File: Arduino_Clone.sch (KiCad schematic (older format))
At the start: 11 parts

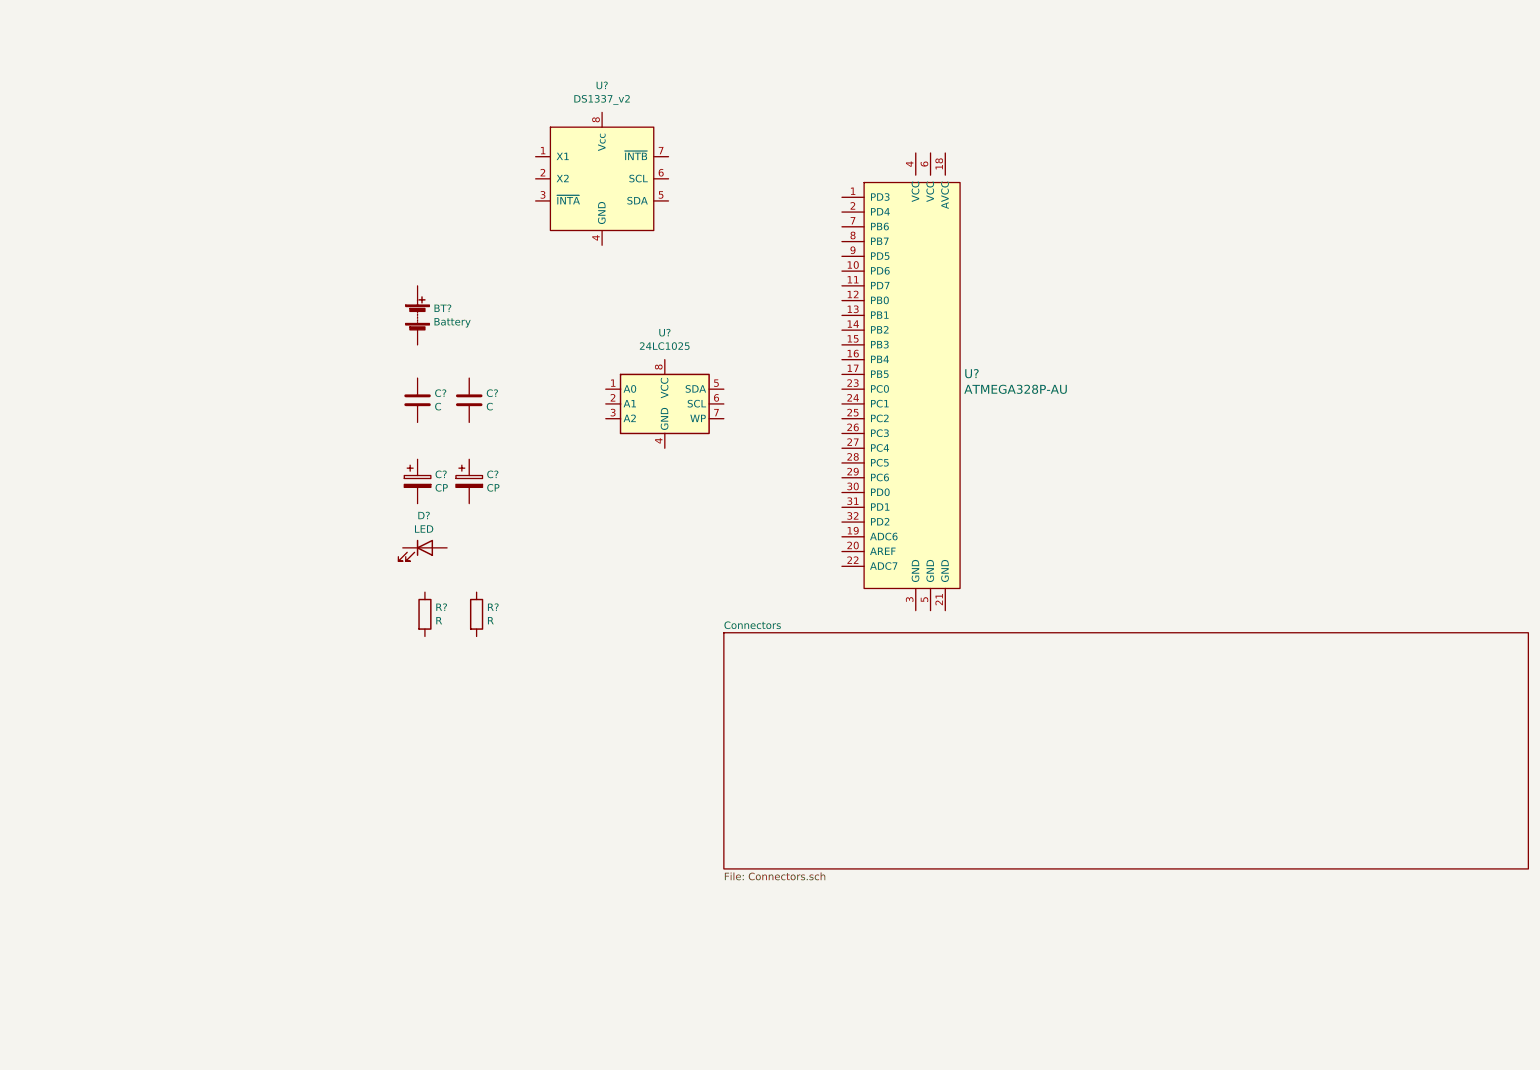
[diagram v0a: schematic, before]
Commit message: Added footprint associations.
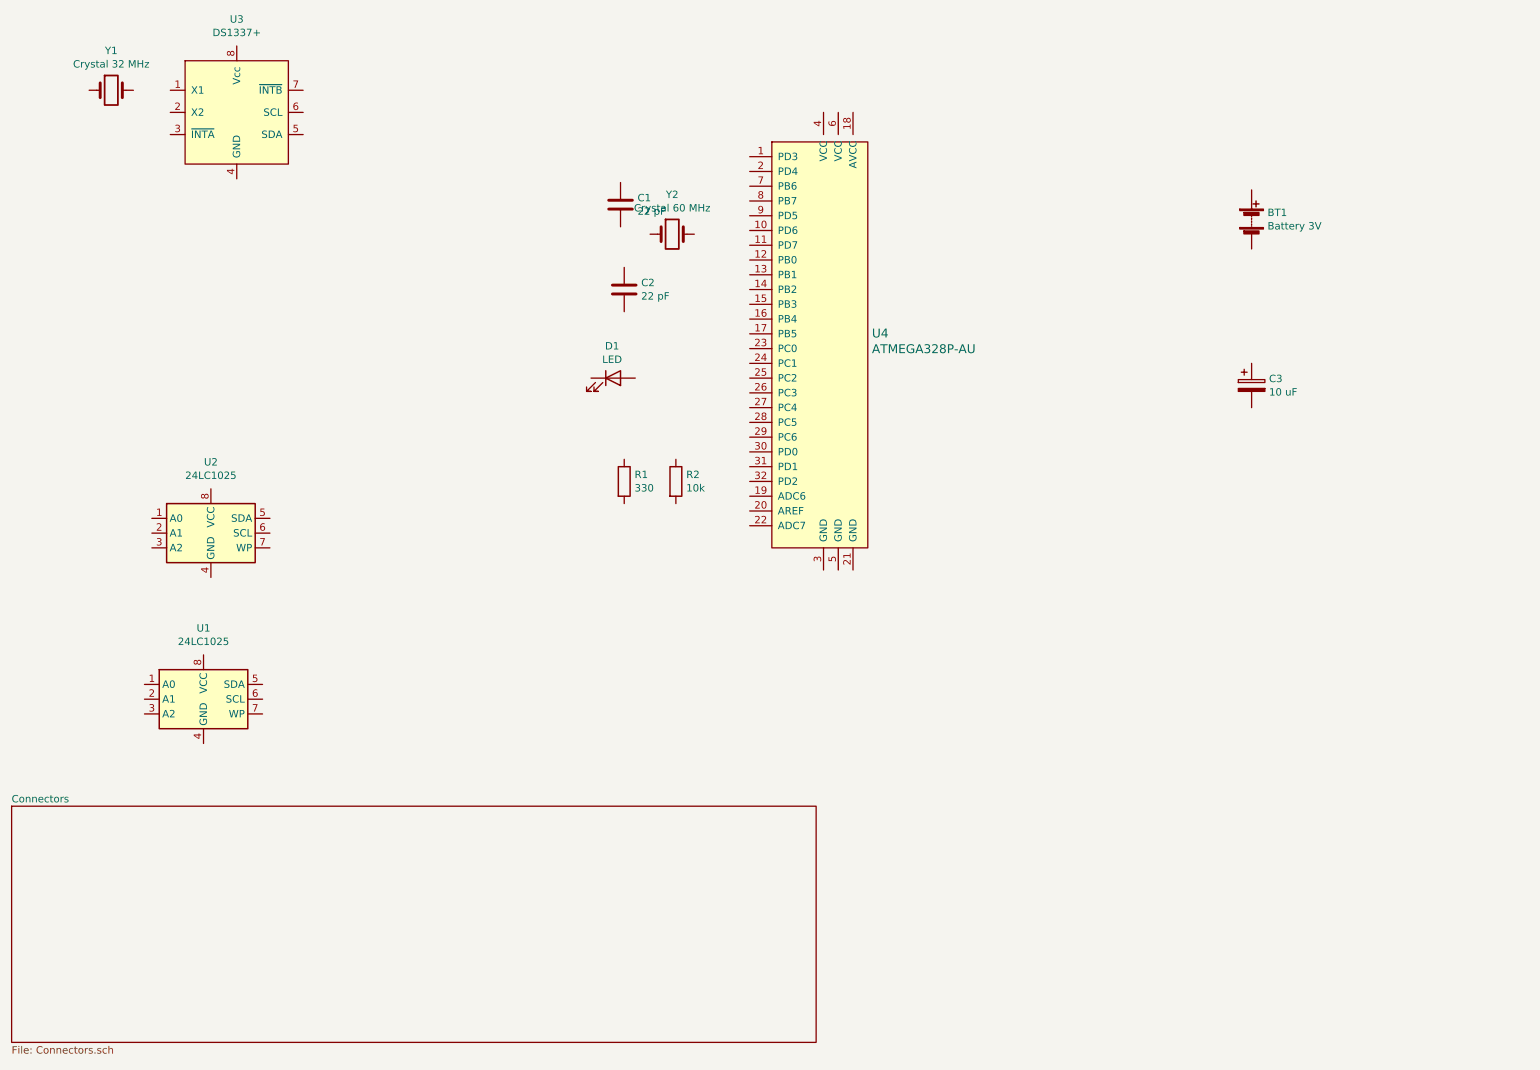
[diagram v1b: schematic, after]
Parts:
- removed C?: CP, symbol Device:CP
- added U2: 24LC1025, Footprints:SOIC-8_3.9mmX4.9mm, symbol Memory_EEPROM:24LC1025
- added Y1: Crystal 32 MHz, Crystal:Crystal_SMD_MicroCrystal_CC7V-T1A-2Pin_3.2x1.5mm_HandSoldering, symbol Device:Crystal
- added Y2: Crystal 60 MHz, Crystal:Crystal_SMD_5032-2Pin_5.0x3.2mm_HandSoldering, symbol Device:Crystal
- BT1: renamed from BT?; value Battery -> Battery 3V; footprint (none) -> Capacitor_SMD:C_0805_2012Metric
- C1, C2: renamed from C?; value C -> 22 pF; footprint (none) -> Capacitor_SMD:C_0805_2012Metric_Pad1.18x1.45mm_HandSolder
- C3: renamed from C?; value CP -> 10 uF; footprint (none) -> Capacitor_SMD:C_0805_2012Metric_Pad1.18x1.45mm_HandSolder
- D1: renamed from D?; footprint (none) -> LED_SMD:LED_0805_2012Metric_Pad1.15x1.40mm_HandSolder
- R1: renamed from R?; value R -> 330; footprint (none) -> Resistor_SMD:R_0805_2012Metric_Pad1.20x1.40mm_HandSolder
- R2: renamed from R?; value R -> 10k; footprint (none) -> Resistor_SMD:R_0805_2012Metric_Pad1.20x1.40mm_HandSolder
- U1: renamed from U?; footprint (none) -> Footprints:SOIC-8_3.9mmX4.9mm
- U3: renamed from U?; value DS1337_v2 -> DS1337+; footprint (none) -> Package_SO:SOIC-8_3.9x4.9mm_P1.27mm
- gave numbers to parts that had none: 1
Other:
- moved on the sheet: BT1, C1, C2, C3, D1, R1, R2, U1, U3, U4
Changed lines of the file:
@@
 $EndDescr
 $Comp
-L Device:Battery BT?
+L Device:Battery BT1
 U 1 1 6016CB0C
-P 3625 2700
-F 0 "BT?" H 3733 2746 50  0000 L CNN
-F 1 "Battery" H 3733 2655 50  0000 L CNN
-F 2 "" V 3625 2760 50  0001 C CNN
-F 3 "~" V 3625 2760 50  0001 C CNN
-	1    3625 2700
+P 9275 2050
+F 0 "BT1" H 9383 2096 50  0000 L CNN
+F 1 "Battery 3V" H 9383 2005 50  0000 L CNN
+F 2 "Capacitor_SMD:C_0805_2012Metric" V 9275 2110 50  0001 C CNN
+F 3 "~" V 9275 2110 50  0001 C CNN
+	1    9275 2050
 	1    0    0    -1
 $EndComp
 $Comp
-L Device:C C?
+L Device:C C1
 U 1 1 6016DE4E
-P 3625 3275
-F 0 "C?" H 3740 3321 50  0000 L CNN
-F 1 "C" H 3740 3230 50  0000 L CNN
-F 2 "" H 3663 3125 50  0001 C CNN
-F 3 "~" H 3625 3275 50  0001 C CNN
-	1    3625 3275
+P 5000 1950
+F 0 "C1" H 5115 1996 50  0000 L CNN
+F 1 "22 pF" H 5115 1905 50  0000 L CNN
+F 2 "Capacitor_SMD:C_0805_2012Metric_Pad1.18x1.45mm_HandSolder" H 5038 1800 50  0001 C CNN
+F 3 "~" H 5000 1950 50  0001 C CNN
+	1    5000 1950
 	1    0    0    -1
 $EndComp
 $Comp
-L Device:C C?
+L Device:C C2
 U 1 1 6016E4DC
-P 3975 3275
-F 0 "C?" H 4090 3321 50  0000 L CNN
-F 1 "C" H 4090 3230 50  0000 L CNN
-F 2 "" H 4013 3125 50  0001 C CNN
-F 3 "~" H 3975 3275 50  0001 C CNN
-	1    3975 3275
+P 5025 2525
+F 0 "C2" H 5140 2571 50  0000 L CNN
+F 1 "22 pF" H 5140 2480 50  0000 L CNN
+F 2 "Capacitor_SMD:C_0805_2012Metric_Pad1.18x1.45mm_HandSolder" H 5063 2375 50  0001 C CNN
+F 3 "~" H 5025 2525 50  0001 C CNN
+	1    5025 2525
 	1    0    0    -1
 $EndComp
 $Comp
-L Device:CP C?
+L Device:CP C3
 U 1 1 6016E8E4
-P 3625 3825
-F 0 "C?" H 3743 3871 50  0000 L CNN
-F 1 "CP" H 3743 3780 50  0000 L CNN
-F 2 "" H 3663 3675 50  0001 C CNN
-F 3 "~" H 3625 3825 50  0001 C CNN
-	1    3625 3825
+P 9275 3175
+F 0 "C3" H 9393 3221 50  0000 L CNN
+F 1 "10 uF" H 9393 3130 50  0000 L CNN
+F 2 "Capacitor_SMD:C_0805_2012Metric_Pad1.18x1.45mm_HandSolder" H 9313 3025 50  0001 C CNN
+F 3 "~" H 9275 3175 50  0001 C CNN
+	1    9275 3175
 	1    0    0    -1
 $EndComp
 $Comp
-L Device:CP C?
-U 1 1 6016ED96
-P 3975 3825
-F 0 "C?" H 4093 3871 50  0000 L CNN
-F 1 "CP" H 4093 3780 50  0000 L CNN
-F 2 "" H 4013 3675 50  0001 C CNN
-F 3 "~" H 3975 3825 50  0001 C CNN
-	1    3975 3825
+L Device:LED D1
+U 1 1 6016F1E9
+P 4950 3125
+F 0 "D1" H 4943 3342 50  0000 C CNN
+F 1 "LED" H 4943 3251 50  0000 C CNN
+F 2 "LED_SMD:LED_0805_2012Metric_Pad1.15x1.40mm_HandSolder" H 4950 3125 50  0001 C CNN
+F 3 "~" H 4950 3125 50  0001 C CNN
+	1    4950 3125
 	1    0    0    -1
 $EndComp
 $Comp
-L Device:LED D?
-U 1 1 6016F1E9
-P 3675 4275
-F 0 "D?" H 3668 4492 50  0000 C CNN
-F 1 "LED" H 3668 4401 50  0000 C CNN
-F 2 "" H 3675 4275 50  0001 C CNN
-F 3 "~" H 3675 4275 50  0001 C CNN
-	1    3675 4275
+L Device:R R1
+U 1 1 6016F7B9
+P 5025 3825
+F 0 "R1" H 5095 3871 50  0000 L CNN
+F 1 "330" H 5095 3780 50  0000 L CNN
+F 2 "Resistor_SMD:R_0805_2012Metric_Pad1.20x1.40mm_HandSolder" V 4955 3825 50  0001 C CNN
+F 3 "~" H 5025 3825 50  0001 C CNN
+	1    5025 3825
 	1    0    0    -1
 $EndComp
 $Comp
-L Device:R R?
-U 1 1 6016F7B9
-P 3675 4725
-F 0 "R?" H 3745 4771 50  0000 L CNN
-F 1 "R" H 3745 4680 50  0000 L CNN
-F 2 "" V 3605 4725 50  0001 C CNN
-F 3 "~" H 3675 4725 50  0001 C CNN
-	1    3675 4725
+L Device:R R2
+U 1 1 6016FC62
+P 5375 3825
+F 0 "R2" H 5445 3871 50  0000 L CNN
+F 1 "10k" H 5445 3780 50  0000 L CNN
+F 2 "Resistor_SMD:R_0805_2012Metric_Pad1.20x1.40mm_HandSolder" V 5305 3825 50  0001 C CNN
+F 3 "~" H 5375 3825 50  0001 C CNN
+	1    5375 3825
 	1    0    0    -1
 $EndComp
 $Comp
-L Device:R R?
-U 1 1 6016FC62
-P 4025 4725
-F 0 "R?" H 4095 4771 50  0000 L CNN
-F 1 "R" H 4095 4680 50  0000 L CNN
-F 2 "" V 3955 4725 50  0001 C CNN
-F 3 "~" H 4025 4725 50  0001 C CNN
-	1    4025 4725
+L Memory_EEPROM:24LC1025 U1
+U 1 1 60170312
+P 2175 5300
+F 0 "U1" H 2175 5781 50  0000 C CNN
+F 1 "24LC1025" H 2175 5690 50  0000 C CNN
+F 2 "Footprints:SOIC-8_3.9mmX4.9mm" H 2175 5300 50  0001 C CNN
+F 3 "http://ww1.microchip.com/downloads/en/DeviceDoc/21941B.pdf" H 2175 5300 50  0001 C CNN
+	1    2175 5300
 	1    0    0    -1
 $EndComp
 $Comp
-L Memory_EEPROM:24LC1025 U?
-U 1 1 60170312
-P 5300 3300
-F 0 "U?" H 5300 3781 50  0000 C CNN
-F 1 "24LC1025" H 5300 3690 50  0000 C CNN
-F 2 "" H 5300 3300 50  0001 C CNN
-F 3 "http://ww1.microchip.com/downloads/en/DeviceDoc/21941B.pdf" H 5300 3300 50  0001 C CNN
-	1    5300 3300
-	1    0    0    -1
-$EndComp
-$Comp
-L dk_Embedded-Microcontrollers:ATMEGA328P-AU U?
+L dk_Embedded-Microcontrollers:ATMEGA328P-AU U4
 U 1 1 601716D4
-P 7000 3200
-F 0 "U?" H 7328 3303 60  0000 L CNN
-F 1 "ATMEGA328P-AU" H 7328 3197 60  0000 L CNN
-F 2 "digikey-footprints:TQFP-32_7x7mm" H 7200 3400 60  0001 L CNN
-F 3 "http://www.microchip.com/mymicrochip/filehandler.aspx?ddocname=en608326" H 7200 3500 60  0001 L CNN
-F 4 "ATMEGA328P-AU-ND" H 7200 3600 60  0001 L CNN "Digi-Key_PN"
-F 5 "ATMEGA328P-AU" H 7200 3700 60  0001 L CNN "MPN"
-F 6 "Integrated Circuits (ICs)" H 7200 3800 60  0001 L CNN "Category"
-F 7 "Embedded - Microcontrollers" H 7200 3900 60  0001 L CNN "Family"
-F 8 "http://www.microchip.com/mymicrochip/filehandler.aspx?ddocname=en608326" H 7200 4000 60  0001 L CNN "DK_Datasheet_Link"
-F 9 "/product-detail/en/microchip-technology/ATMEGA328P-AU/ATMEGA328P-AU-ND/1832260" H 7200 4100 60  0001 L CNN "DK_Detail_Page"
-F 10 "IC MCU 8BIT 32KB FLASH 32TQFP" H 7200 4200 60  0001 L CNN "Description"
-F 11 "Microchip Technology" H 7200 4300 60  0001 L CNN "Manufacturer"
-F 12 "Active" H 7200 4400 60  0001 L CNN "Status"
-	1    7000 3200
+P 6375 2925
+F 0 "U4" H 6703 3028 60  0000 L CNN
+F 1 "ATMEGA328P-AU" H 6703 2922 60  0000 L CNN
+F 2 "digikey-footprints:TQFP-32_7x7mm" H 6575 3125 60  0001 L CNN
+F 3 "http://www.microchip.com/mymicrochip/filehandler.aspx?ddocname=en608326" H 6575 3225 60  0001 L CNN
+F 4 "ATMEGA328P-AU-ND" H 6575 3325 60  0001 L CNN "Digi-Key_PN"
+F 5 "ATMEGA328P-AU" H 6575 3425 60  0001 L CNN "MPN"
+F 6 "Integrated Circuits (ICs)" H 6575 3525 60  0001 L CNN "Category"
+F 7 "Embedded - Microcontrollers" H 6575 3625 60  0001 L CNN "Family"
+F 8 "http://www.microchip.com/mymicrochip/filehandler.aspx?ddocname=en608326" H 6575 3725 60  0001 L CNN "DK_Datasheet_Link"
+F 9 "/product-detail/en/microchip-technology/ATMEGA328P-AU/ATMEGA328P-AU-ND/1832260" H 6575 3825 60  0001 L CNN "DK_Detail_Page"
+F 10 "IC MCU 8BIT 32KB FLASH 32TQFP" H 6575 3925 60  0001 L CNN "Description"
+F 11 "Microchip Technology" H 6575 4025 60  0001 L CNN "Manufacturer"
+F 12 "Active" H 6575 4125 60  0001 L CNN "Status"
+	1    6375 2925
 	1    0    0    -1
 $EndComp
 $Sheet
-S 5700 4850 5450 1600
+S 875  6025 5450 1600
 U 6017416D
 F0 "Connectors" 50
@@
 $EndSheet
 $Comp
-L My_Library:DS1337_v2 U?
+L My_Library:DS1337_v2 U3
 U 1 1 6017BB22
-P 4875 1775
-F 0 "U?" H 4875 2406 50  0000 C CNN
-F 1 "DS1337_v2" H 4875 2315 50  0000 C CNN
-F 2 "" H 4925 1825 50  0001 C CNN
-F 3 "https://datasheets.maximintegrated.com/en/ds/DS1337-DS1337C.pdf" H 4925 1825 50  0001 C CNN
-	1    4875 1775
+P 2400 1325
+F 0 "U3" H 2400 1956 50  0000 C CNN
+F 1 "DS1337+" H 2400 1865 50  0000 C CNN
+F 2 "Package_SO:SOIC-8_3.9x4.9mm_P1.27mm" H 2450 1375 50  0001 C CNN
+F 3 "https://datasheets.maximintegrated.com/en/ds/DS1337-DS1337C.pdf" H 2450 1375 50  0001 C CNN
+	1    2400 1325
 	1    0    0    -1
 $EndComp
+$Comp
+L Device:Crystal Y1
+U 1 1 6017D062
+P 1550 1175
+F 0 "Y1" H 1550 1443 50  0000 C CNN
+F 1 "Crystal 32 MHz" H 1550 1352 50  0000 C CNN
+F 2 "Crystal:Crystal_SMD_MicroCrystal_CC7V-T1A-2Pin_3.2x1.5mm_HandSoldering" H 1550 1175 50  0001 C CNN
+F 3 "~" H 1550 1175 50  0001 C CNN
+	1    1550 1175
+	1    0    0    -1
+$EndComp
+$Comp
+L Device:Crystal Y2
+U 1 1 6017DF24
+P 5350 2150
+F 0 "Y2" H 5350 2418 50  0000 C CNN
+F 1 "Crystal 60 MHz" H 5350 2327 50  0000 C CNN
+F 2 "Crystal:Crystal_SMD_5032-2Pin_5.0x3.2mm_HandSoldering" H 5350 2150 50  0001 C CNN
+F 3 "~" H 5350 2150 50  0001 C CNN
+	1    5350 2150
+	1    0    0    -1
+$EndComp
+$Comp
+L Memory_EEPROM:24LC1025 U2
+U 1 1 6018204D
+P 2225 4175
+F 0 "U2" H 2225 4656 50  0000 C CNN
+F 1 "24LC1025" H 2225 4565 50  0000 C CNN
+F 2 "Footprints:SOIC-8_3.9mmX4.9mm" H 2225 4175 50  0001 C CNN
+F 3 "http://ww1.microchip.com/downloads/en/DeviceDoc/21941B.pdf" H 2225 4175 50  0001 C CNN
+	1    2225 4175
+	1    0    0    -1
+$EndComp
